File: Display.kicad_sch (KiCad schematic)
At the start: 3 parts, among them U4 X1000, U8 M25PX32-VMW, U9 TFP410PAP

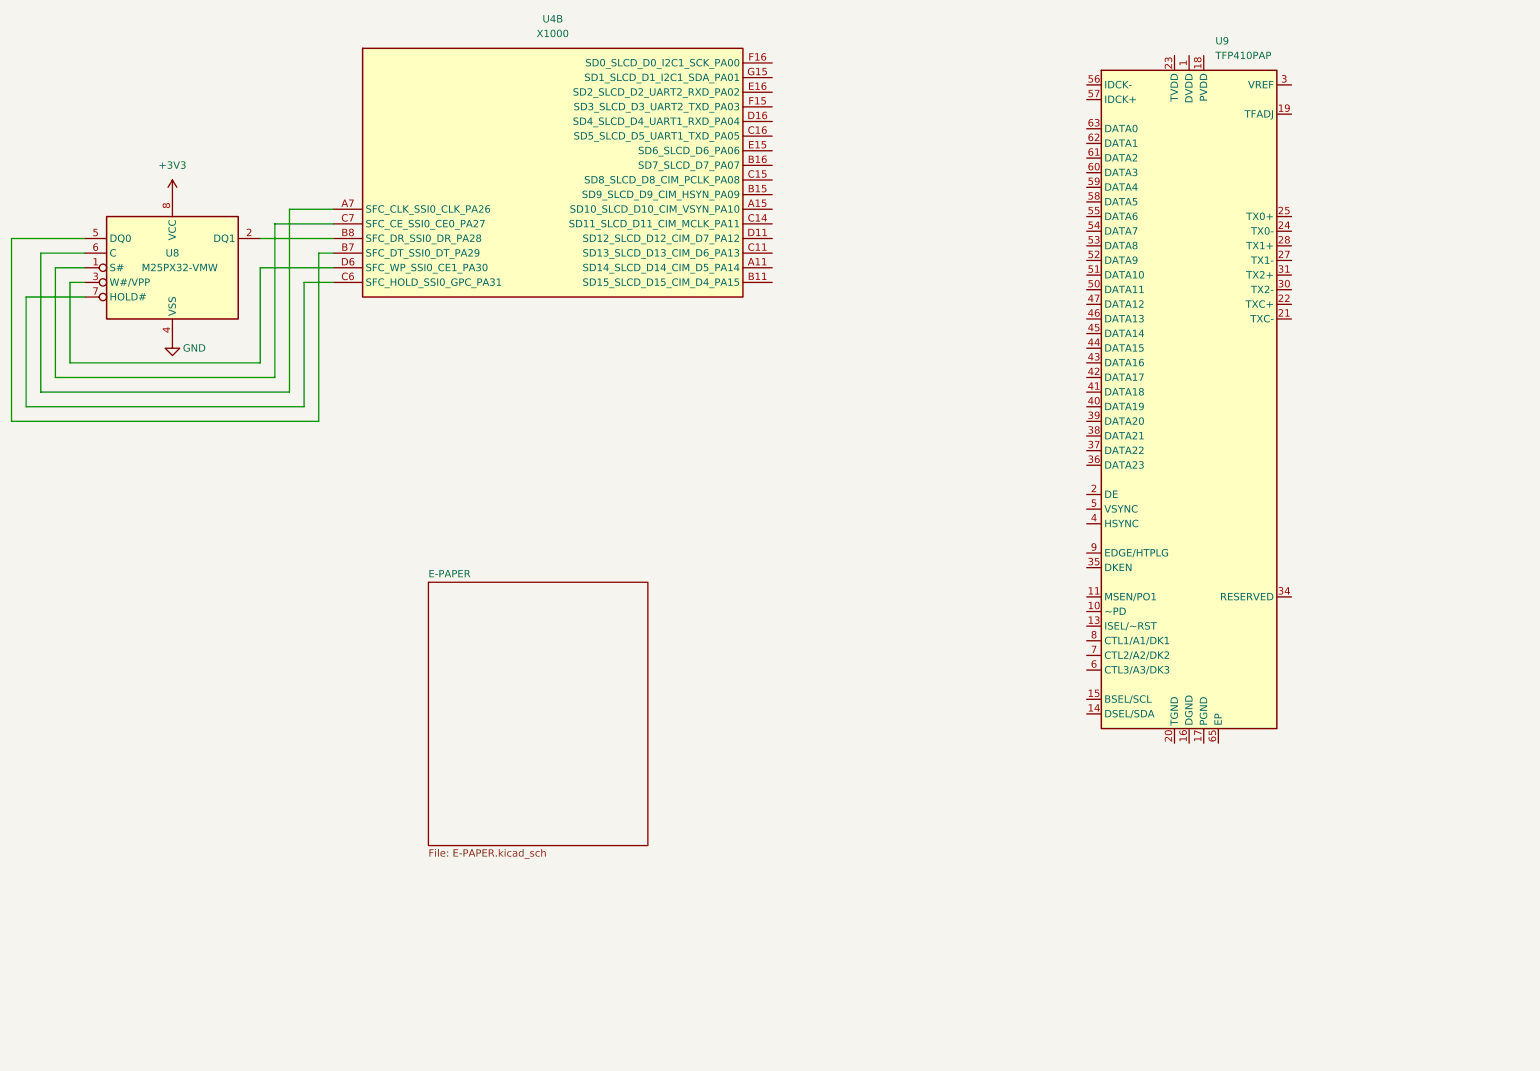
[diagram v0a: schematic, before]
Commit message: Update (Display)
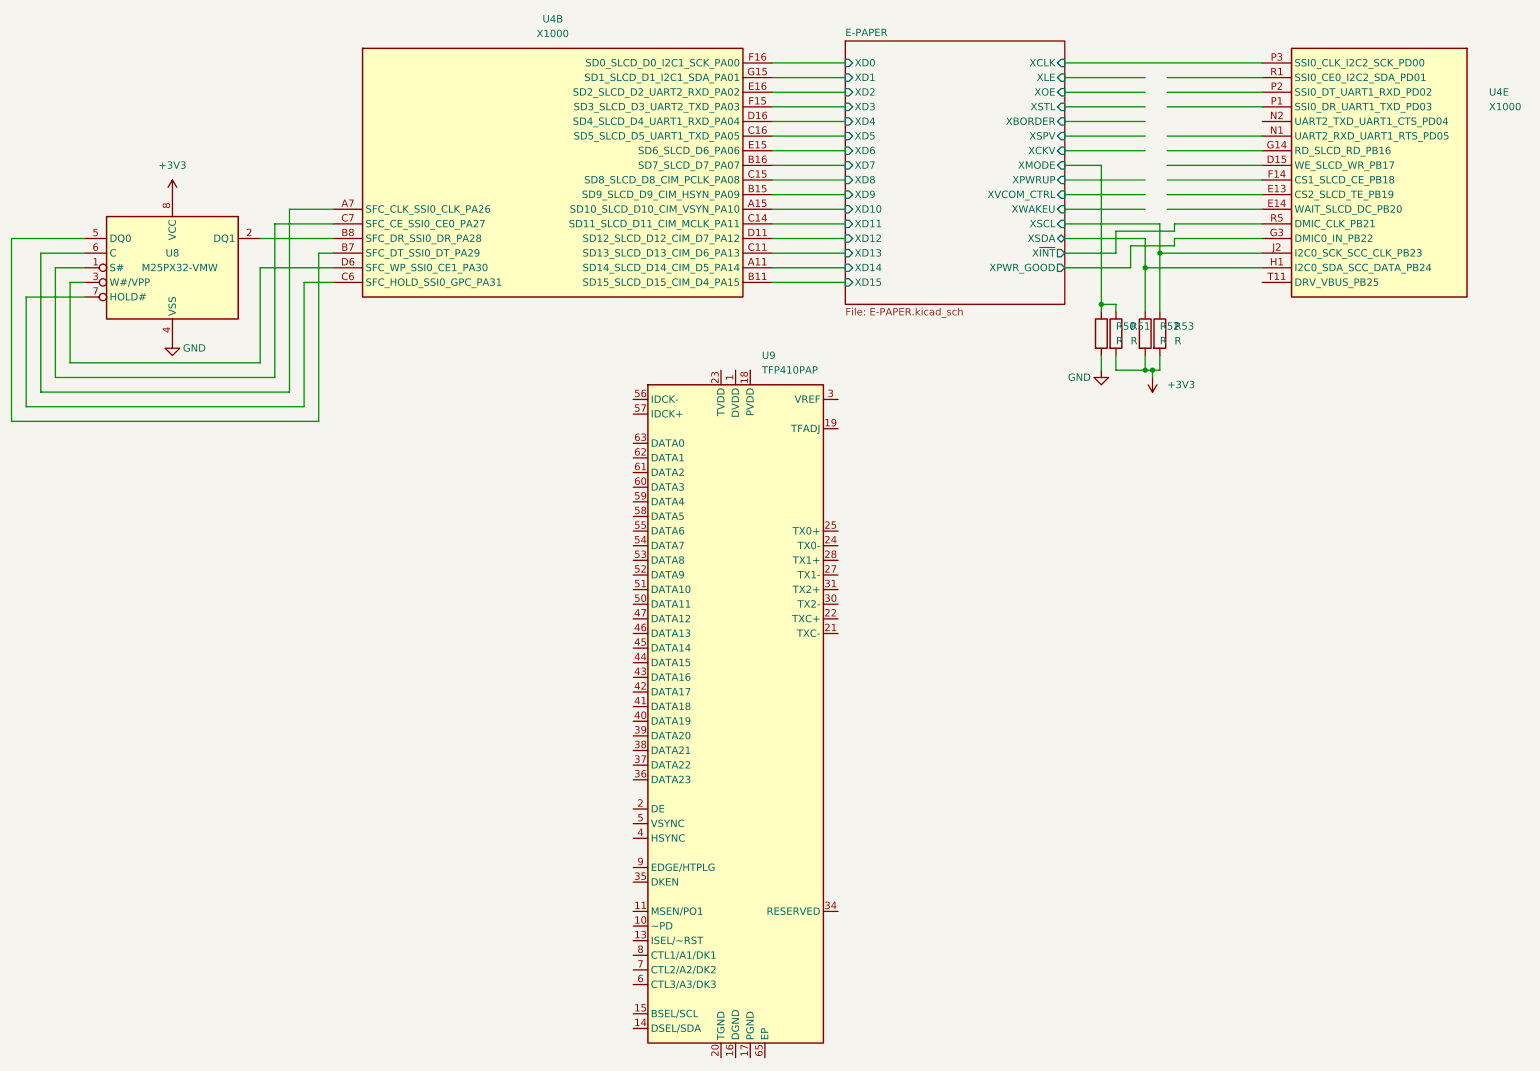
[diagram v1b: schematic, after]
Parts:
- added R50, R51, R52, R53: R, symbol Device:R
- added unit 5 of U4
- U4: footprint (none) -> TheBrutzlers_Lib:BGA256C80P16X16_1300X1300X130N
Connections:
- net +3V3: now also R51.2, R52.2, R53.2
- net GND: now also R50.2
- net E-PAPER/XD14: now reaches U4.A11 (SD14_SLCD_D14_CIM_D5_PA14)
- net E-PAPER/XD10: now reaches U4.A15 (SD10_SLCD_D10_CIM_VSYN_PA10)
- net E-PAPER/XD15: now reaches U4.B11 (SD15_SLCD_D15_CIM_D4_PA15)
- net E-PAPER/XD9: now reaches U4.B15 (SD9_SLCD_D9_CIM_HSYN_PA09)
- net E-PAPER/XD7: now reaches U4.B16 (SD7_SLCD_D7_PA07)
- net E-PAPER/XD13: now reaches U4.C11 (SD13_SLCD_D13_CIM_D6_PA13)
- net E-PAPER/XD11: now reaches U4.C14 (SD11_SLCD_D11_CIM_MCLK_PA11)
- net E-PAPER/XD8: now reaches U4.C15 (SD8_SLCD_D8_CIM_PCLK_PA08)
- net E-PAPER/XD5: now reaches U4.C16 (SD5_SLCD_D5_UART1_TXD_PA05)
- net E-PAPER/XD12: now reaches U4.D11 (SD12_SLCD_D12_CIM_D7_PA12)
- net E-PAPER/XD4: now reaches U4.D16 (SD4_SLCD_D4_UART1_RXD_PA04)
- net E-PAPER/XD6: now reaches U4.E15 (SD6_SLCD_D6_PA06)
- net E-PAPER/XD2: now reaches U4.E16 (SD2_SLCD_D2_UART2_RXD_PA02)
- net E-PAPER/XD3: now reaches U4.F15 (SD3_SLCD_D3_UART2_TXD_PA03)
- net E-PAPER/XD0: now reaches U4.F16 (SD0_SLCD_D0_I2C1_SCK_PA00)
- net E-PAPER/XD1: now reaches U4.G15 (SD1_SLCD_D1_I2C1_SDA_PA01)
- new net E-PAPER/XCLK: U4.P3 (SSI0_CLK_I2C2_SCK_PD00)
- new net E-PAPER/XMODE: R50.1, R51.1
- new net E-PAPER/XPWR_GOOD: U4.G3 (DMIC0_IN_PB22)
- new net E-PAPER/XSCL: R53.1, U4.J2 (I2C0_SCK_SCC_CLK_PB23)
- new net E-PAPER/XSDA: R52.1, U4.H1 (I2C0_SDA_SCC_DATA_PB24)
- new net E-PAPER/X~{INT}: U4.R5 (DMIC_CLK_PB21)
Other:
- sheet E-PAPER ports: added XBORDER, XCKV, XCLK, XD0, XD1, XD10, XD11, XD12, XD13, XD14, XD15, XD2, XD3, XD4, XD5, XD6, XD7, XD8, XD9, XLE, XMODE, XOE, XPWRUP, XPWR_GOOD, XSCL, XSDA, XSPV, XSTL, XVCOM_CTRL, XWAKEU, X~{INT}; removed none
- moved on the sheet: U9
